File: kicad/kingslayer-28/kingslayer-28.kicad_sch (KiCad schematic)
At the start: 57 parts, among them K1 KEYSW, K10 KEYSW, K11 KEYSW, K12 KEYSW, K13 KEYSW, K14 KEYSW, K15 KEYSW, K16 KEYSW, K17 KEYSW, K18 KEYSW, K19 KEYSW, K2 KEYSW, K20 KEYSW, K21 KEYSW, K22 KEYSW, K23 KEYSW, K24 KEYSW, K25 KEYSW, K26 KEYSW, K27 KEYSW, K28 KEYSW, K3 KEYSW, K4 KEYSW, K5 KEYSW, K6 KEYSW, K7 KEYSW, K8 KEYSW, K9 KEYSW, U1 STM32F303CCTx

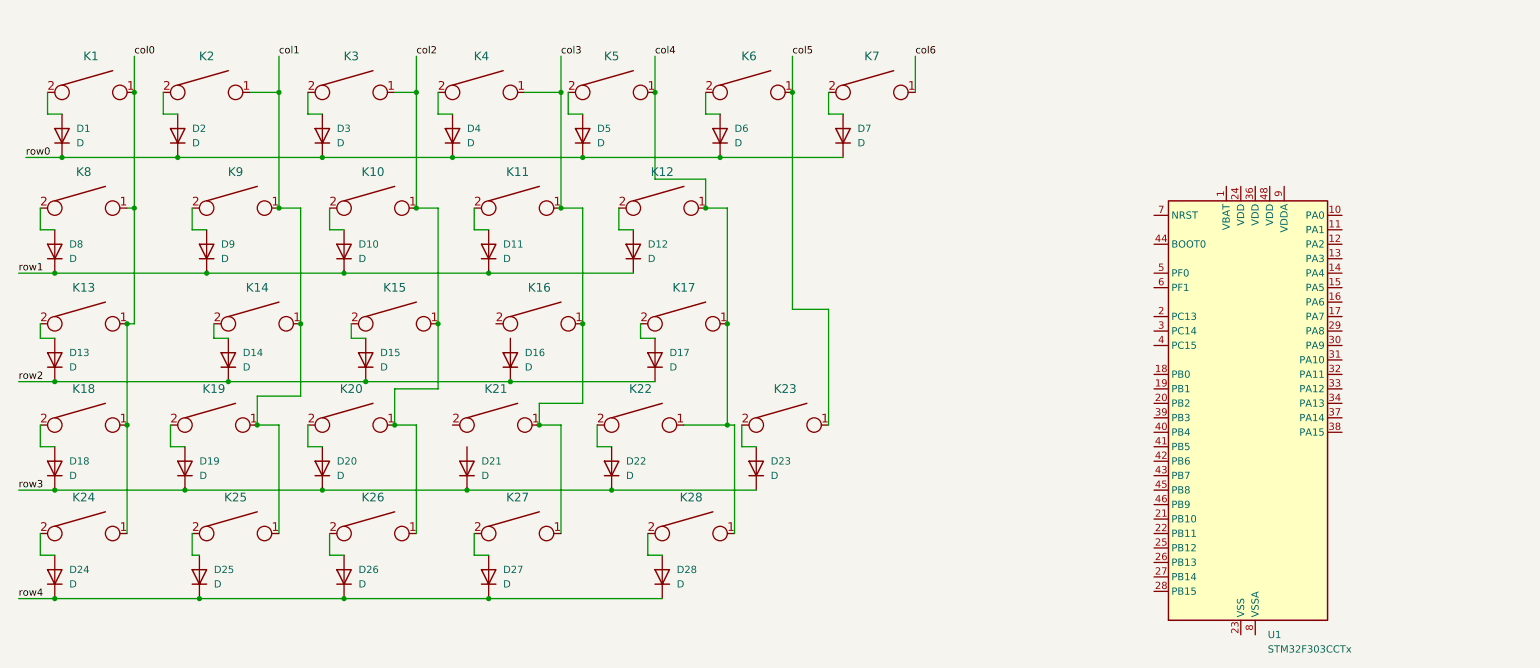
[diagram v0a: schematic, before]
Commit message: Setting up microcontroller
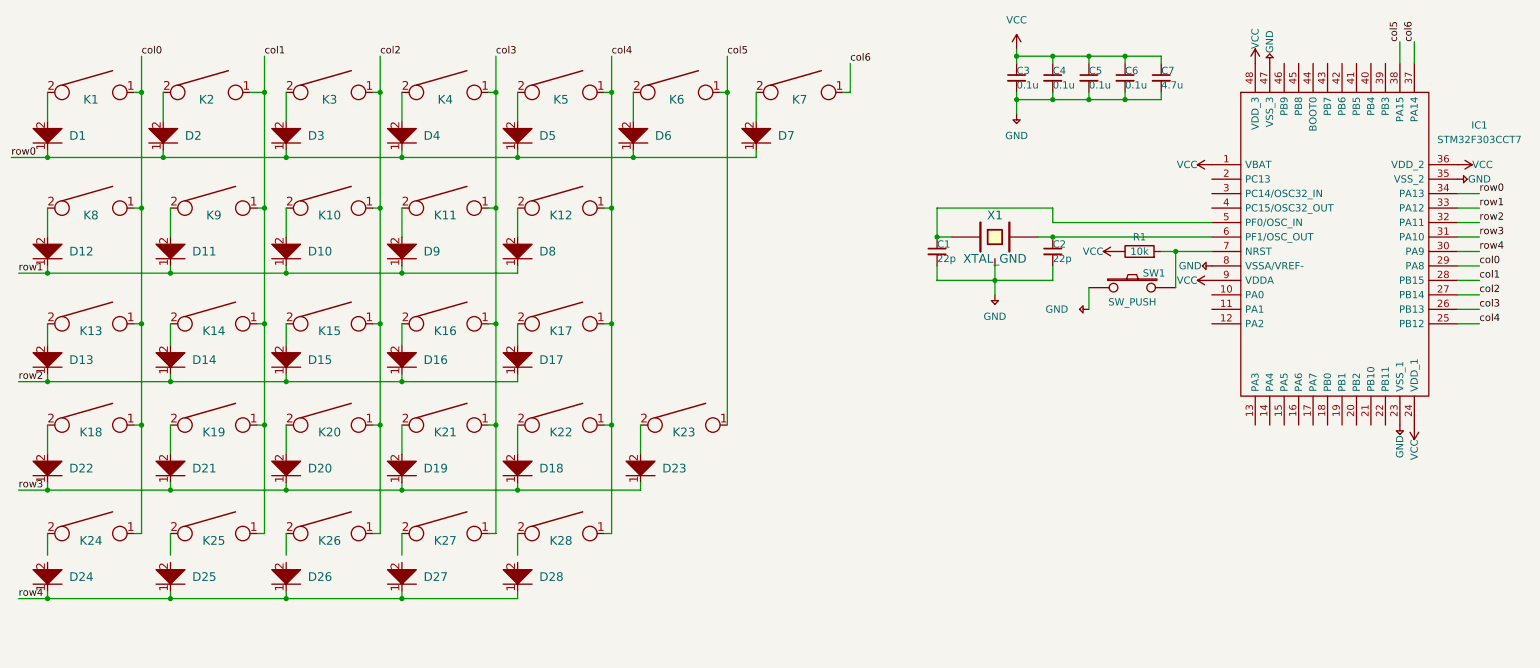
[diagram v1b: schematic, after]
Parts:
- removed D1, D10, D11, D12, D13, D14, D15, D16, D17, D18, D19, D2, D20, D21, D22, D23, D24, D25, D26, D27, D28, D3, D4, D5, D6, D7, D8, D9: D, symbol Device:D
- removed U1: STM32F303CCTx, Package_QFP:LQFP-48_7x7mm_P0.5mm, symbol MCU_ST_STM32F3:STM32F303CCTx
- added C1, C2: 22p, symbol Device:C_Small
- added C3, C4, C5, C6: 0.1u, symbol Device:C_Small
- added C7: 4.7u, symbol Device:C_Small
- added D1, D10, D11, D12, D13, D14, D15, D16, D17, D18, D19, D2, D20, D21, D22, D23, D24, D25, D26, D27, D28, D3, D4, D5, D6, D7, D8, D9: D, symbol keyboard_parts:D
- added IC1: STM32F303CCT7, QFP50P900X900X160-48N, symbol STM32F303CCT7:STM32F303CCT7
- added R1: 10k, symbol Device:R
- added SW1: SW_PUSH, symbol keyboard_parts:SW_PUSH
- added X1: XTAL_GND, symbol keyboard_parts:XTAL_GND
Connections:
- net col0: now also IC1.29 (PA8)
- net col1: now also IC1.28 (PB15)
- net col2: now also IC1.27 (PB14)
- net col3: now also IC1.26 (PB13)
- net col4: now also IC1.25 (PB12)
- net col5: now also IC1.38 (PA15)
- net col6: now also IC1.37 (PA14)
- net row0: now also D1.1, D2.1, D3.1, D4.1, D5.1, D6.1, D7.1, IC1.34 (PA13)
- net row1: now also D10.1, D11.1, D12.1, D8.1, D9.1, IC1.33 (PA12)
- net row2: now also D13.1, D14.1, D15.1, D16.1, D17.1, IC1.32 (PA11)
- net row3: now also D18.1, D19.1, D20.1, D21.1, D22.1, D23.1, IC1.31 (PA10)
- net row4: now also D24.1, D25.1, D26.1, D27.1, D28.1, IC1.30 (PA9)
- net at K15.2: now also D15.2
- net at K12.2: now also D8.2
- net at K7.2: now also D7.2
- net at K17.2: now also D17.2
- net at K9.2: now also D11.2
- net at K1.2: now also D1.2
- net at K18.2: now also D22.2
- net at K13.2: now also D13.2
- net at K19.2: now also D21.2
- net at K20.2: now also D20.2
- net at K3.2: now also D3.2
- net at K5.2: now also D5.2
- net at K11.2: now also D9.2
- net at K14.2: now also D14.2
- net at K16.2: now also D16.2
- net at K21.2: now also D19.2
- net at K22.2: now also D18.2
- net at K2.2: now also D2.2
- net at K8.2: now also D12.2
- net at K4.2: now also D4.2
- net at K10.2: now also D10.2
- net at K23.2: now also D23.2
- net at K6.2: now also D6.2
- new net: C1.1, IC1.5 (PF0/OSC_IN), X1.1
- new net: C2.1, IC1.6 (PF1/OSC_OUT), X1.2
- new net: IC1.7 (NRST), R1.2, SW1.2
- new net +5V: C1.2, C2.2, C3.2, C4.2, C5.2, C6.2, C7.2, IC1.23 (VSS_1), IC1.35 (VSS_2), IC1.47 (VSS_3), IC1.8 (VSSA/VREF-), SW1.1, X1.3
- new net VCC: C3.1, C4.1, C5.1, C6.1, C7.1, IC1.1 (VBAT), IC1.24 (VDD_1), IC1.36 (VDD_2), IC1.48 (VDD_3), IC1.9 (VDDA), R1.1
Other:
- moved on the sheet: K10, K11, K12, K13, K14, K15, K16, K17, K18, K20, K21, K22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
